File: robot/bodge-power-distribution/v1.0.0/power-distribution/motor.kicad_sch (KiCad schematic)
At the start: 17 parts, among them J10 1053082204, J11 1053082204, J12 1053072202, J13 1053072202, J14 1053082204, J15 1053082204, J16 1053072202, J17 1053072202, J18 MOTOR_{BRUSHED}, J19 RS1-03-G, J6 1053082204, J7 1053082204, J8 1053072202, J9 1053072202, U7 DRV8220

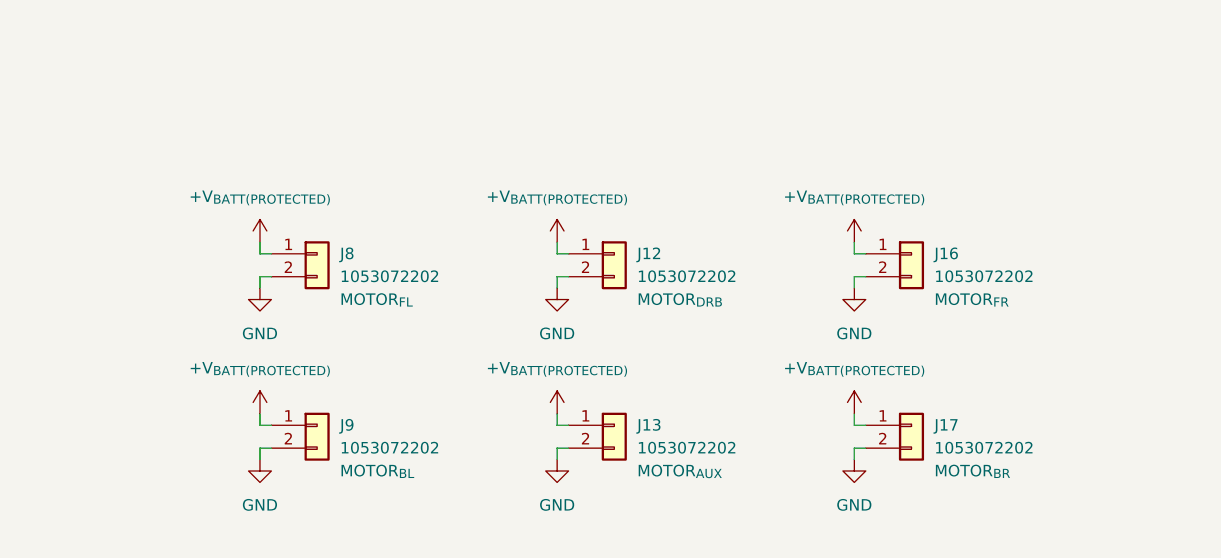
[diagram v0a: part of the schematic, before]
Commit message: Post-review updates
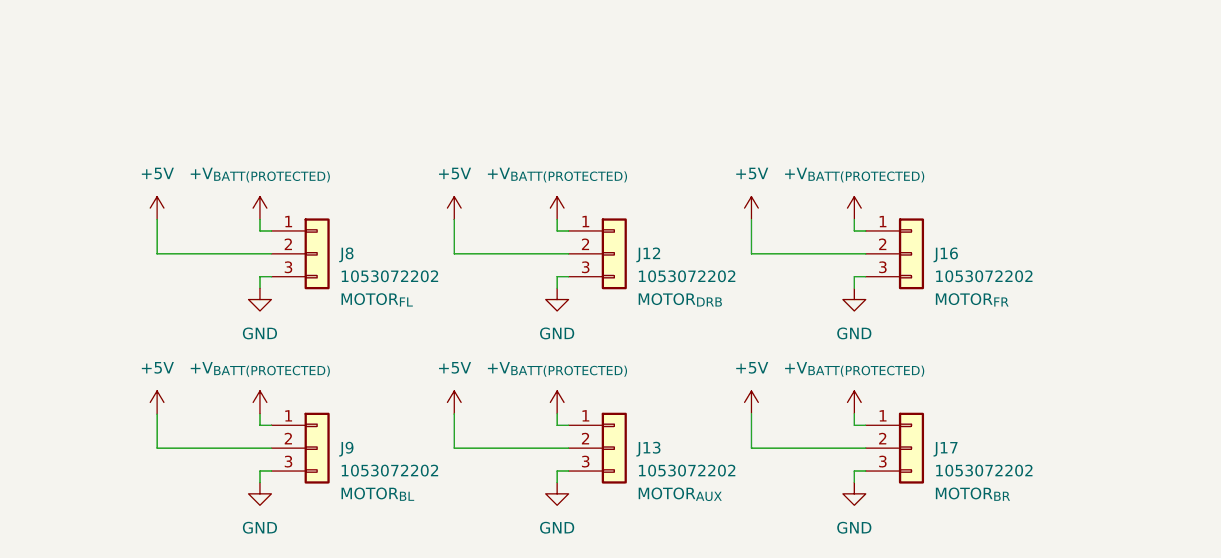
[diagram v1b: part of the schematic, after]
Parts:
- J12, J13, J16, J17, J8, J9: footprint AT-Connectors:1x02_P3mm_3x5mm_Plug_SMD -> AT-Connectors:1x03_P3mm_ID0.8mm_OD2mm_Plug_TH; symbol Connector_Generic:Conn_01x02 -> Connector_Generic:Conn_01x03
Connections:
- net +5V: now also J12.2 (Pin_2), J13.2 (Pin_2), J16.2 (Pin_2), J17.2 (Pin_2), J8.2 (Pin_2), J9.2 (Pin_2)
- net GND: now also J12.3 (Pin_3), J13.3 (Pin_3), J16.3 (Pin_3), J17.3 (Pin_3), J8.3 (Pin_3), J9.3 (Pin_3); no longer J12.2 (Pin_2), J13.2 (Pin_2), J16.2 (Pin_2), J17.2 (Pin_2), J8.2 (Pin_2), J9.2 (Pin_2)
